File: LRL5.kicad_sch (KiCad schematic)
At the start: 38 parts, among them J1 POWER, J2 On/Off, J5 OUT, J6 MODE, J7 ADJUST, Q1 BC549, U1 BA033CC0T, U2 NHD-C0220BIZ

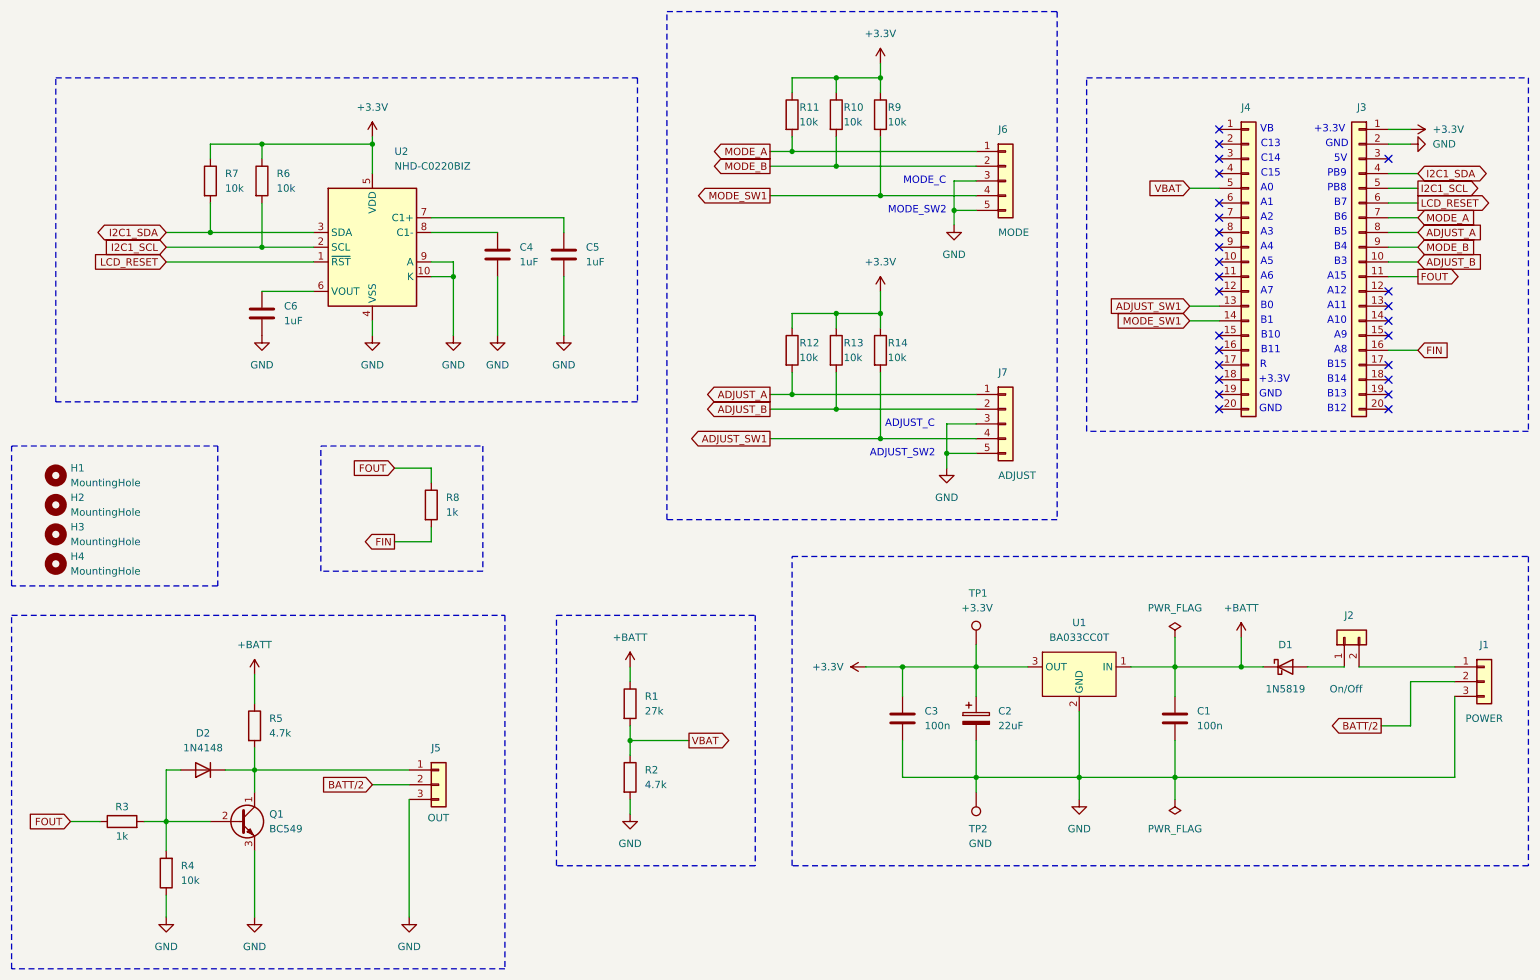
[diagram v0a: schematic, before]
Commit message: Some PCB optimizations 1
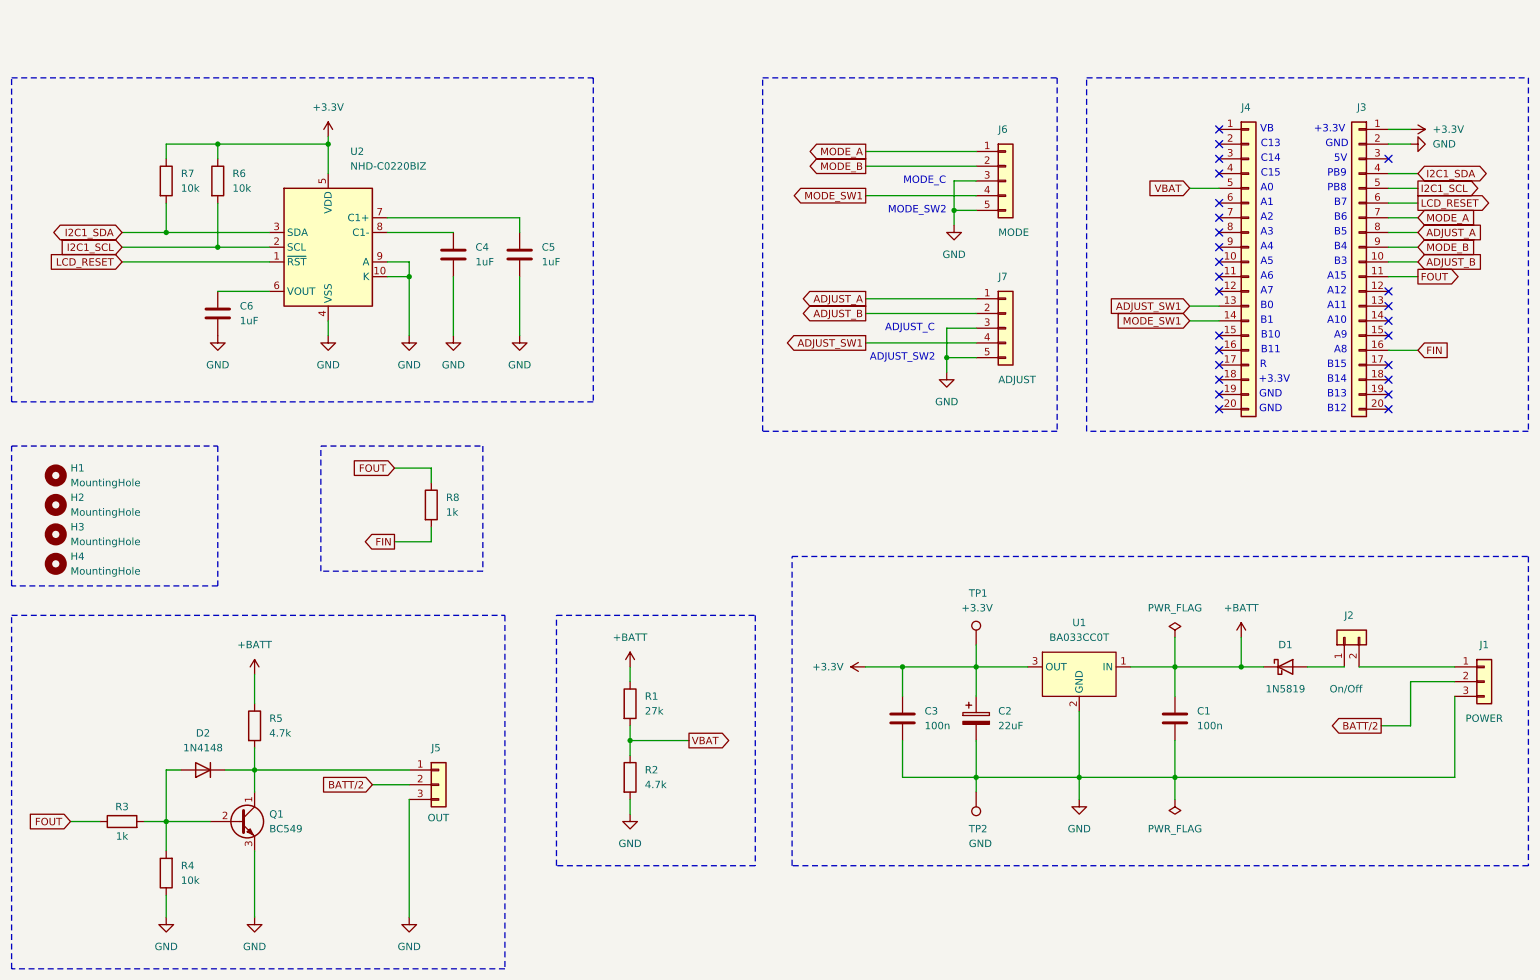
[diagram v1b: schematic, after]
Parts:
- removed R10, R11, R12, R13, R14, R9: 10k, Resistor_SMD:R_0805_2012Metric_Pad1.20x1.40mm_HandSolder, symbol Device:R
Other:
- moved on the sheet: C4, C5, C6, J7, R6, R7, U2
